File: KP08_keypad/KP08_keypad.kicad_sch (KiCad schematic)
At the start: 15 parts, among them J1 Conn_01x13, J2 Conn_01x13, J3 Conn_01x03, SW1 SW_Push, SW10 SW_Push_SPDT, SW11 SW_Push, SW12 SW_Push_SPDT, SW2 SW_Push, SW3 SW_Push, SW4 SW_Push, SW5 SW_Push, SW6 SW_Push, SW7 SW_Push, SW8 SW_Push, SW9 SW_Push

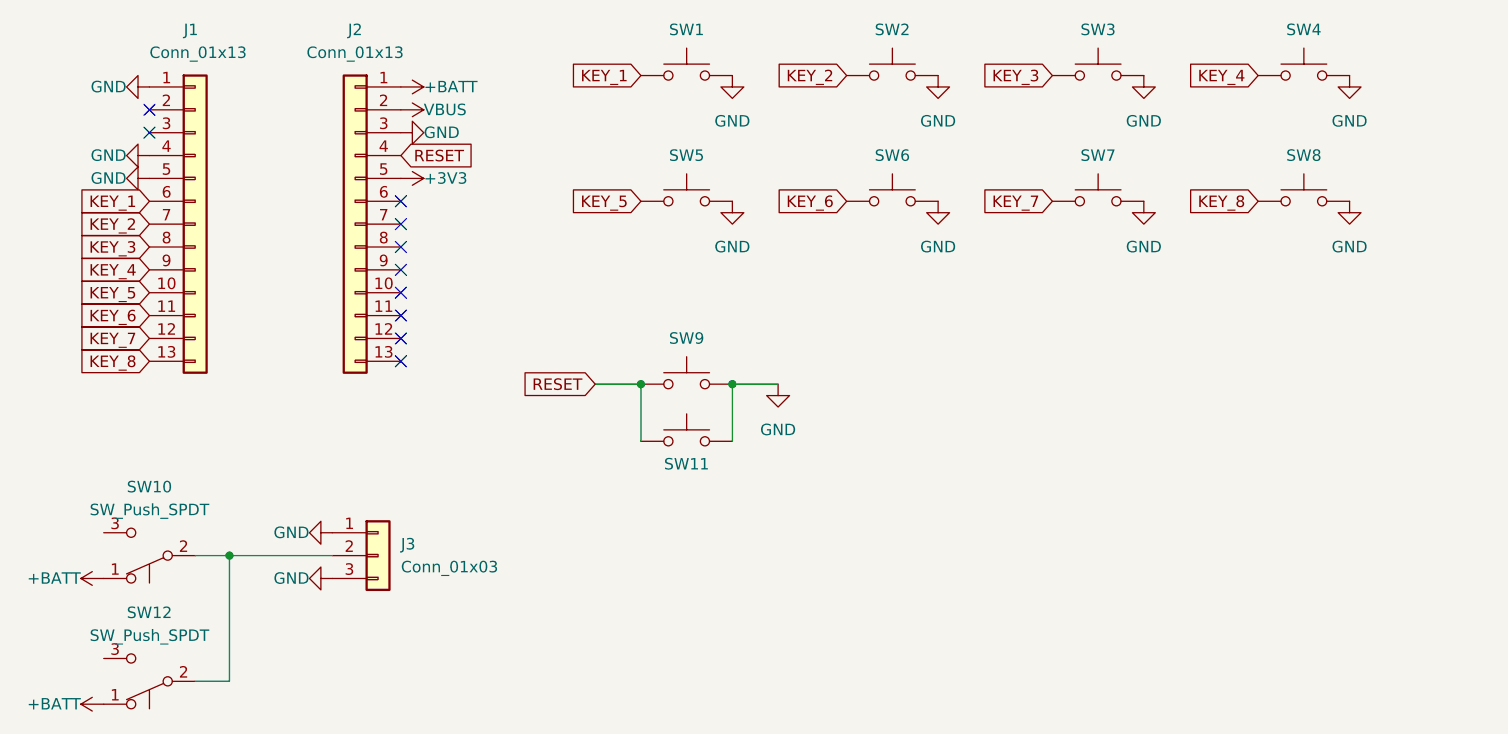
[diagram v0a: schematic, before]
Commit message: Update footprint
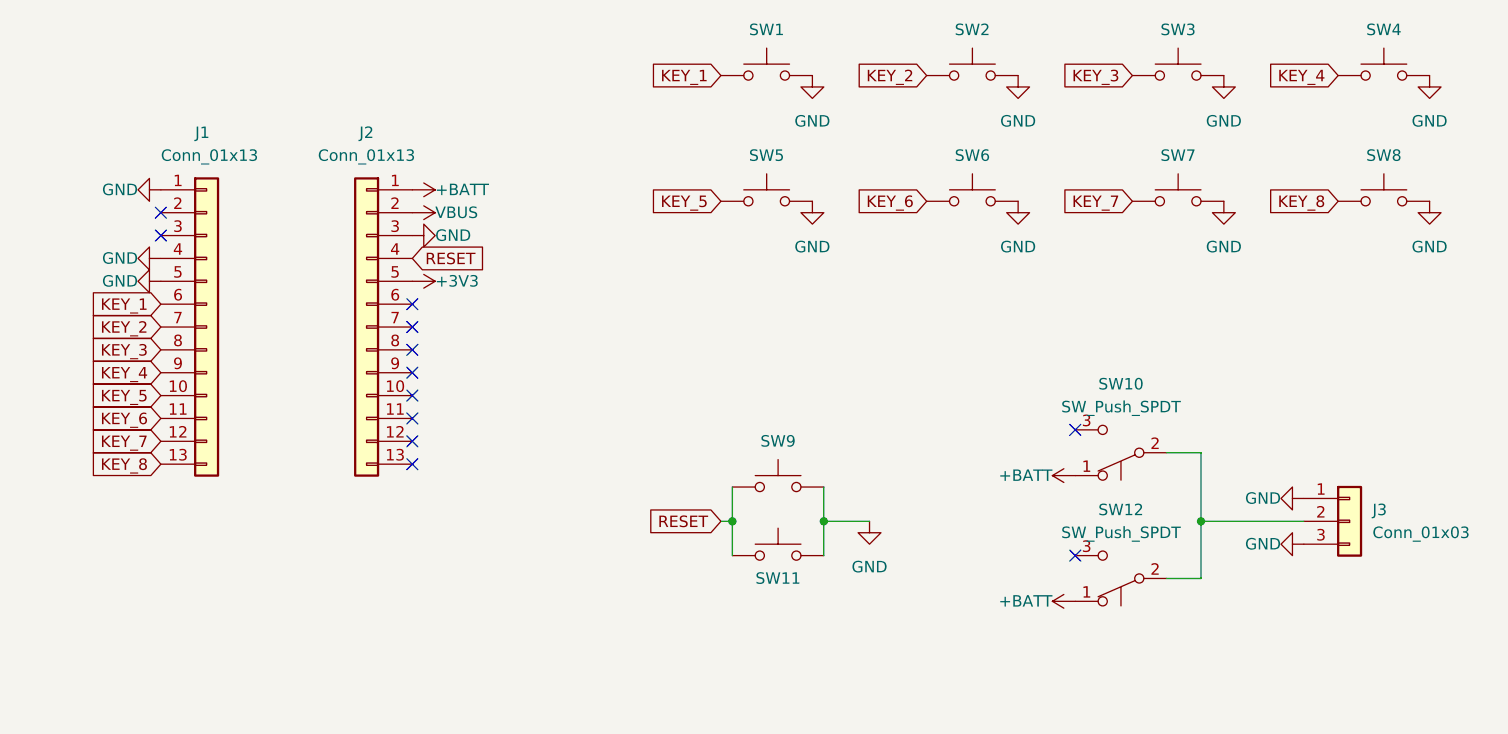
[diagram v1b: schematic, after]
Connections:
- no-connect marks 10 -> 12
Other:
- moved on the sheet: J1, J2, J3, SW1, SW10, SW11, SW12, SW2, SW3, SW4, SW5, SW6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
